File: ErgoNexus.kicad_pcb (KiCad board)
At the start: 2 copper layers, 185.4 x 144.3 mm, 130 parts, among them J10 Conn_01x06, J7 Conn_01x02, J8 Conn_01x02, J9 Conn_01x06, SW1 SW_Push, SW2 RotaryEncoder_Switch, SW3 SW_Push, SW4 RotaryEncoder_Switch, U1 SuperMini nRF52840, U2 SuperMini nRF52840

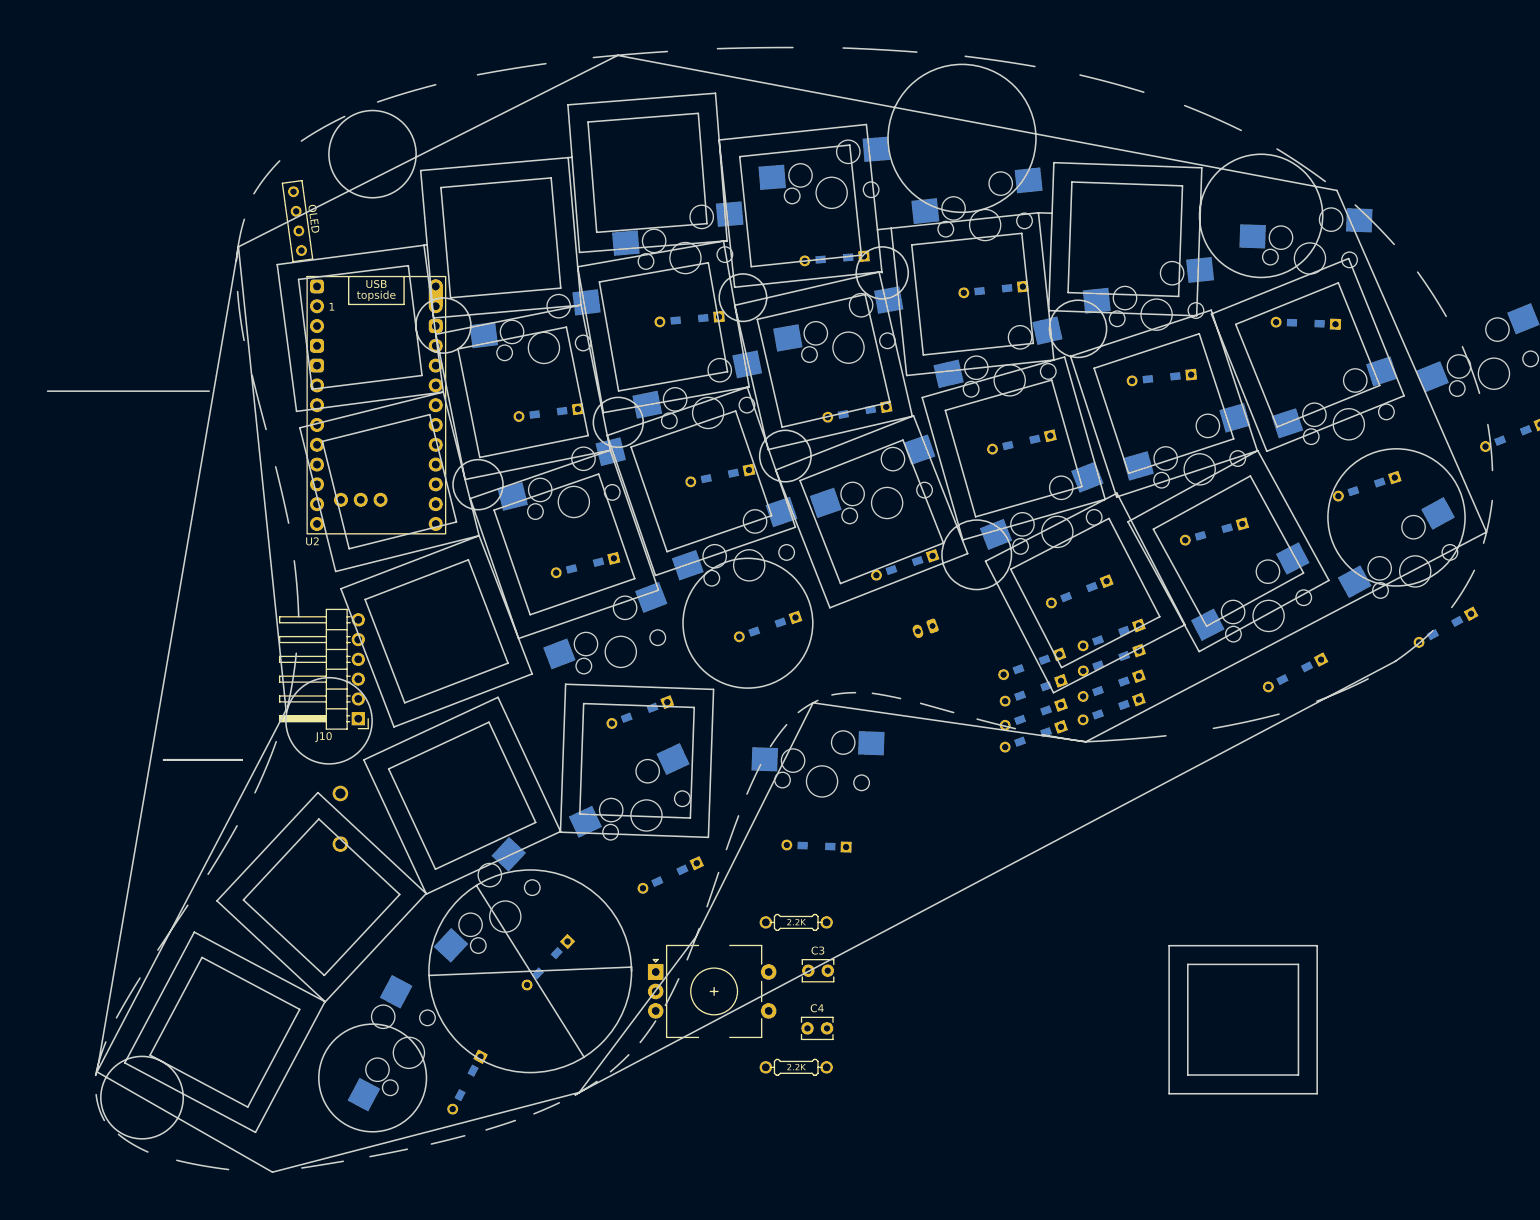
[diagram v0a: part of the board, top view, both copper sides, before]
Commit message: chore: remove Cuts
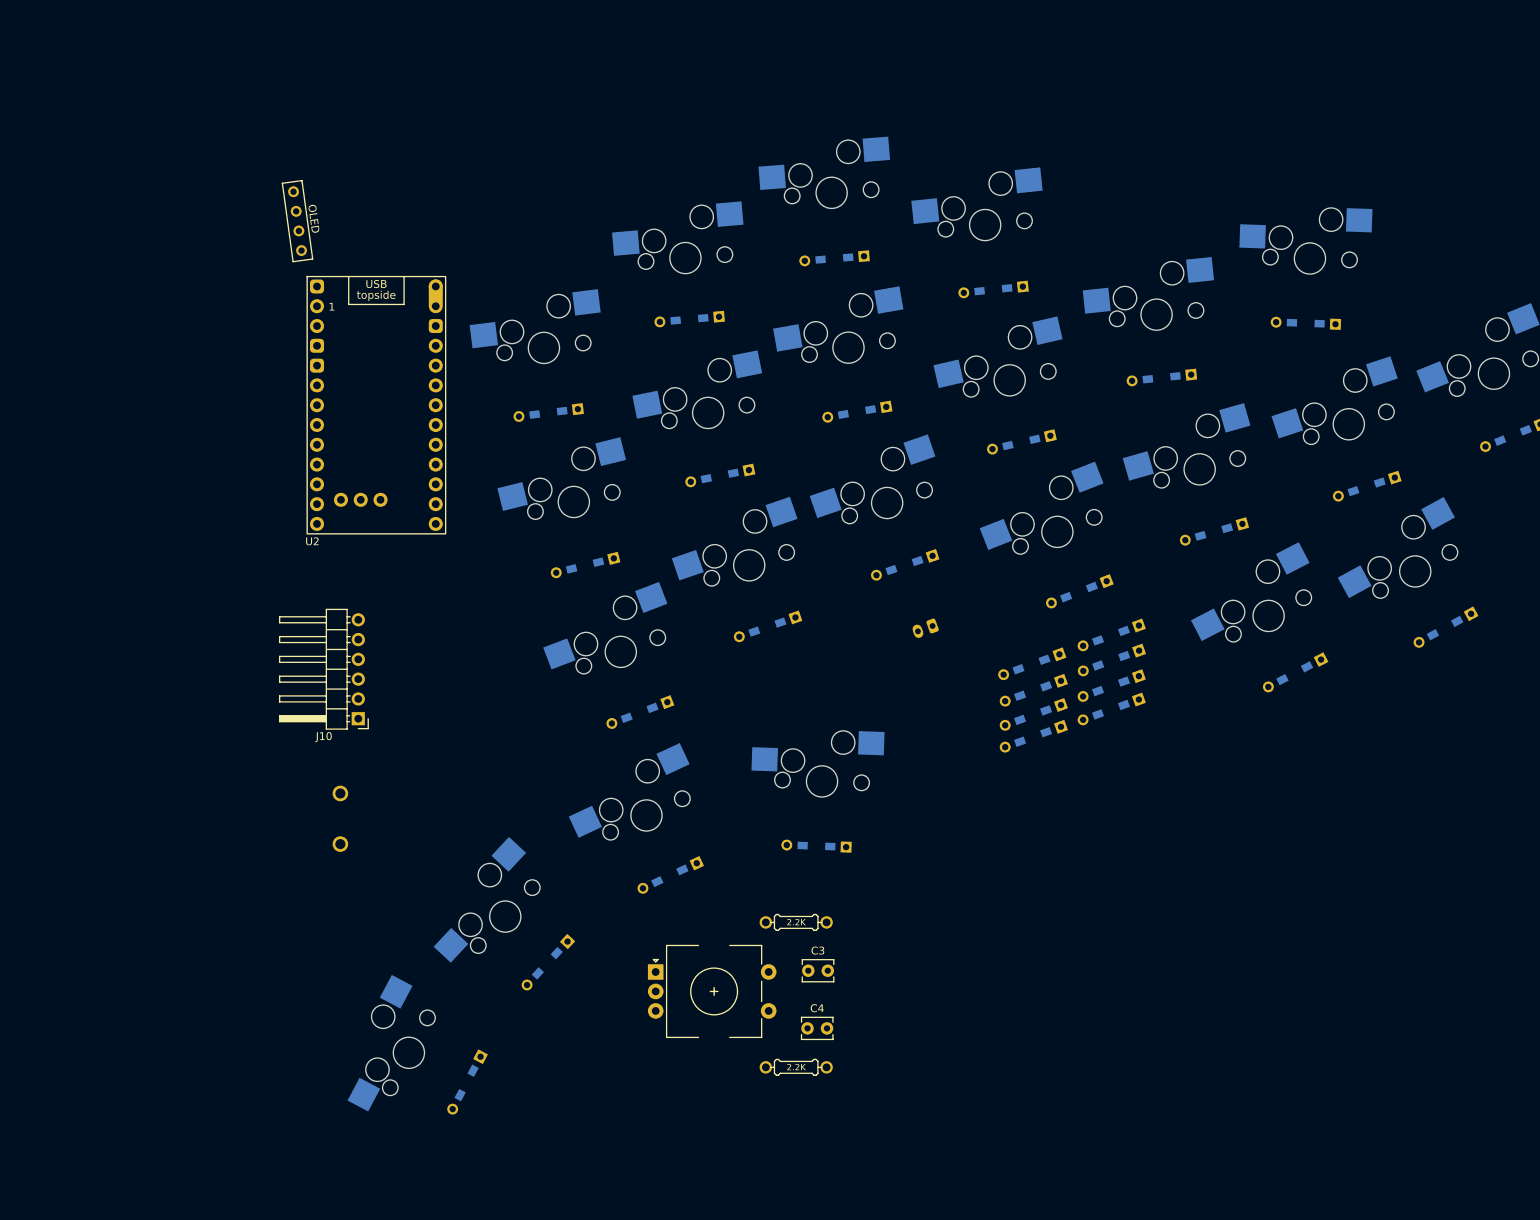
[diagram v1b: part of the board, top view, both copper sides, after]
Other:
- board outline removed
